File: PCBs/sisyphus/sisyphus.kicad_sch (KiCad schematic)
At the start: 65 parts, among them J1 USB_C_Receptacle_USB2.0_14P, J2 AUX USB, J3 Conn_01x02, J4 Speaker, J5 SWD, J6 RGB_CONN, J7 Keyboard, J8 Light sensor, J9 Battery, U1 NCP1117-3.3_SOT223, U2 USBLC6-2P6, U3 W25Q128JVS, U4 MAX98357A, U5 RP2040, U7 BQ25619, Y1 ABM8-272-T3

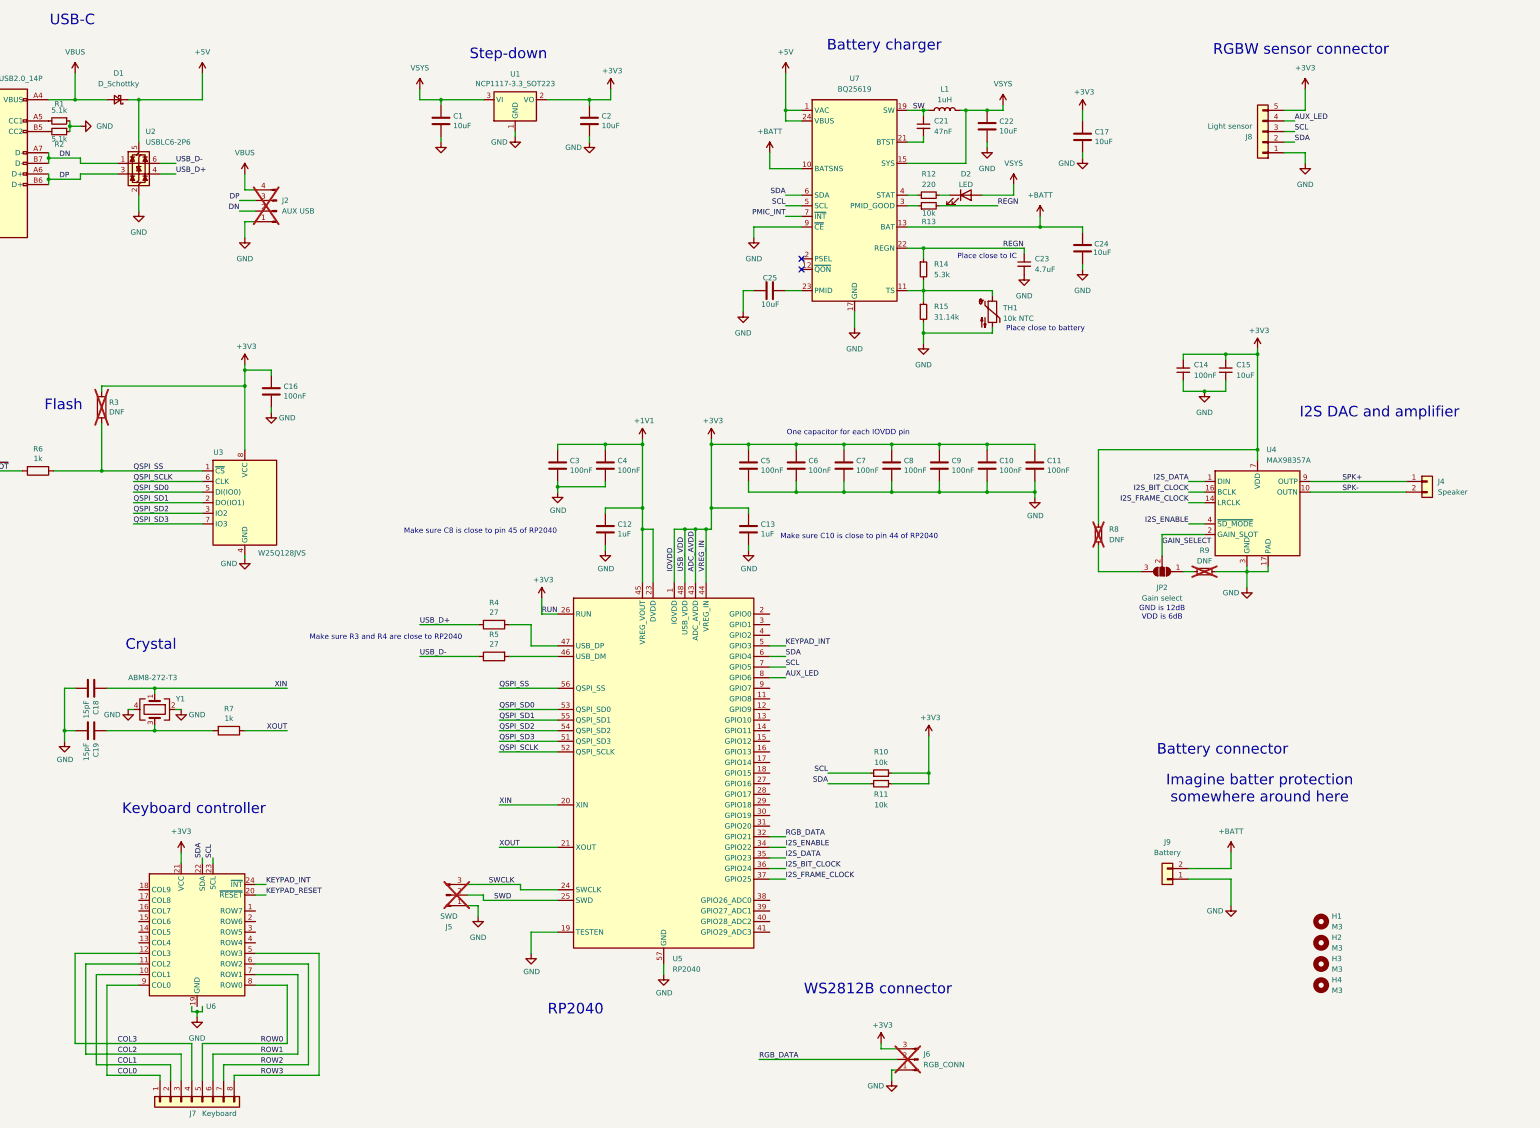
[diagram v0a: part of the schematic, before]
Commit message: Major PCB update
I won't even bother commenting it
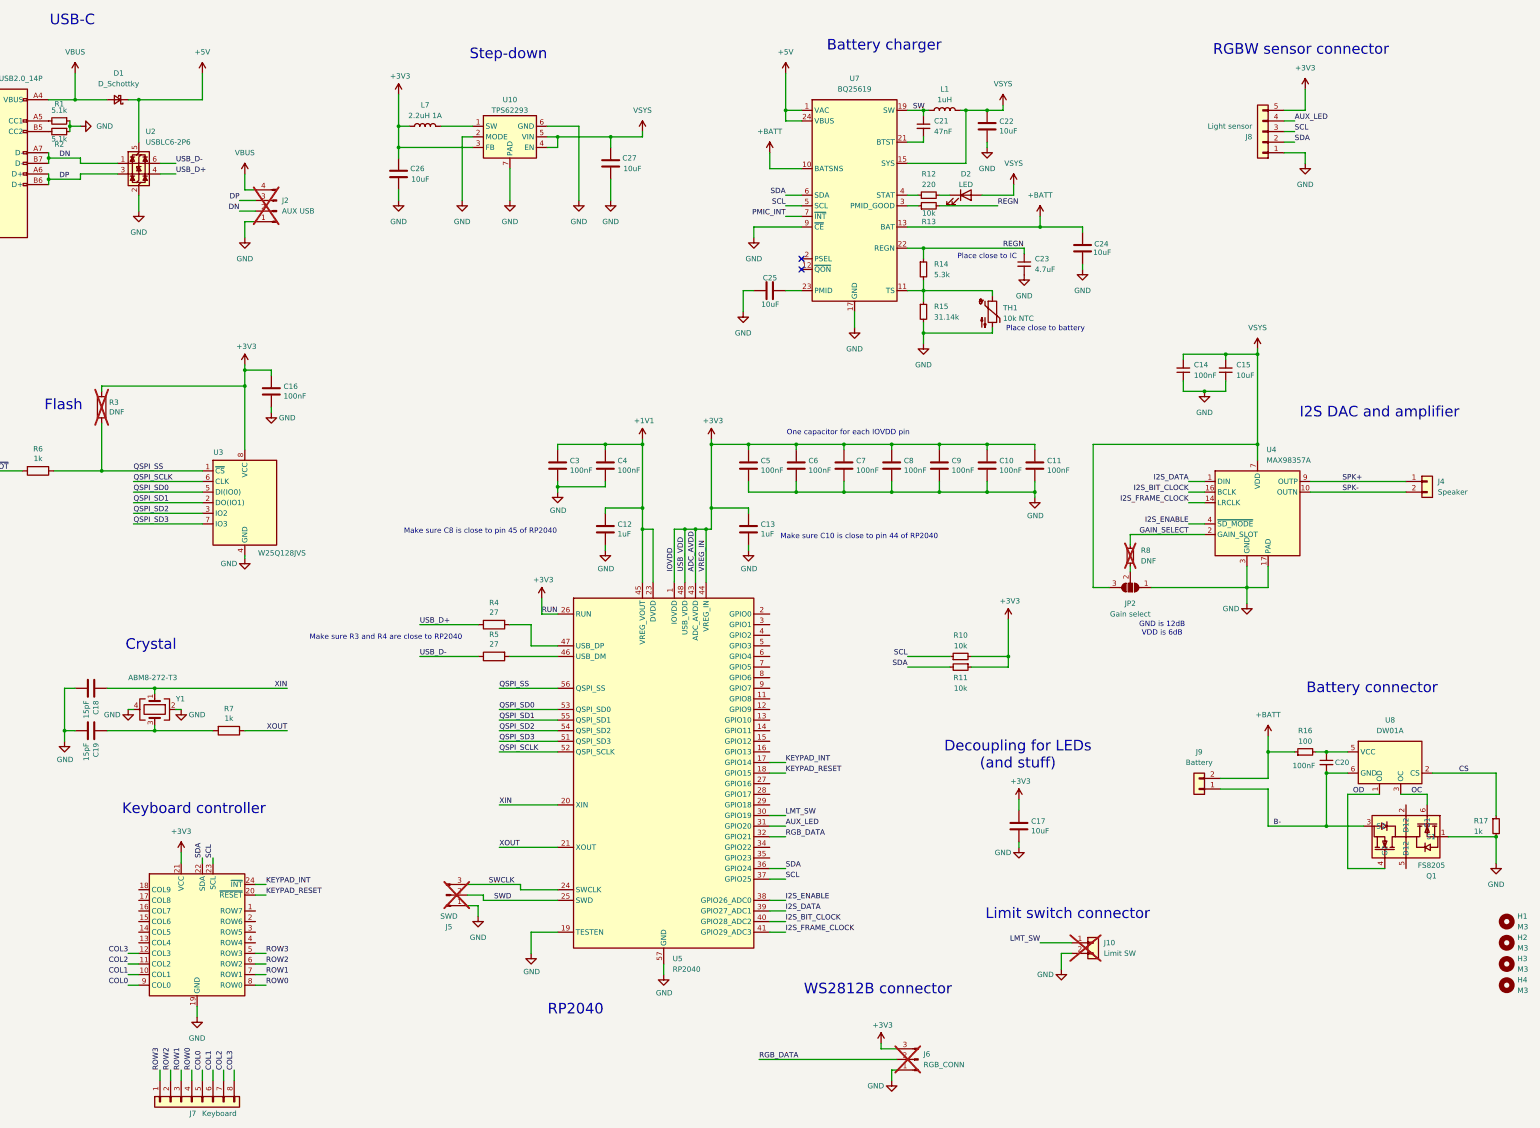
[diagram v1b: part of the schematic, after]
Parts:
- removed C1, C2: 10uF, Capacitor_SMD:C_0805_2012Metric, symbol Device:C
- removed R9: DNF, Resistor_SMD:R_0402_1005Metric, symbol Device:R_Small
- removed U1: NCP1117-3.3_SOT223, Package_TO_SOT_SMD:SOT-223-3_TabPin2, symbol Regulator_Linear:NCP1117-3.3_SOT223
- added C20: 100nF, Capacitor_SMD:C_0402_1005Metric, symbol Device:C_Small
- added C26, C27: 10uF, Capacitor_SMD:C_0402_1005Metric, symbol Device:C
- added J10: Limit SW, Connector_PinSocket_2.54mm:PinSocket_1x02_P2.54mm_Vertical, symbol Connector_Generic:Conn_01x02
- added L7: 2.2uH 1A, Inductor_SMD:L_0603_1608Metric, symbol Device:L
- added Q1: FS8205, Package_TO_SOT_SMD:SOT-23-6, symbol easyeda2kicad:FS8205
- added R16: 100, Resistor_SMD:R_0402_1005Metric, symbol Device:R_Small
- added R17: 1k, Resistor_SMD:R_0402_1005Metric, symbol Device:R_Small
- added U10: TPS62293, Package_SON:WSON-6-1EP_2x2mm_P0.65mm_EP1x1.6mm_ThermalVias, symbol Sisyphus:TPS62293
- added U8: DW01A, Package_TO_SOT_SMD:SOT-23-6, symbol Battery_Management:DW01A
- C15, C17, C22, C24, C25: footprint Capacitor_SMD:C_0805_2012Metric -> Capacitor_SMD:C_0402_1005Metric
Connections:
- net +3V3: now also C26.1, L7.1, U10.3 (FB); no longer C14.2, C15.2, R8.1, U4.7 (VDD), U4.8 (VDD)
- net +BATT: now also R16.1
- net AUX_LED: now also U5.31 (GPIO20); no longer U5.8 (GPIO6)
- net COL0: now also J7.5 (Pin_5); no longer J7.1 (Pin_1)
- net COL1: now also J7.6 (Pin_6); no longer J7.2 (Pin_2)
- net COL2: now also J7.7 (Pin_7); no longer J7.3 (Pin_3)
- net COL3: now also J7.8 (Pin_8); no longer J7.4 (Pin_4)
- net GAIN_SELECT: now also R8.1; no longer JP2.2 (C)
- net GND: now also JP2.1 (A), U6.19 (GND), U6.25 (PAD), C26.2, C27.2, J10.2 (Pin_2), Q1.1 (S1), R17.2, U10.2 (MODE), U10.6 (GND), U10.7 (PAD); no longer J9.1 (Pin_1)
- net I2S_BIT_CLOCK: now also U5.40 (GPIO28_ADC2); no longer U5.36 (GPIO24)
- net I2S_DATA: now also U5.39 (GPIO27_ADC1); no longer U5.35 (GPIO23)
- net I2S_ENABLE: now also U5.38 (GPIO26_ADC0); no longer U5.34 (GPIO22)
- net I2S_FRAME_CLOCK: now also U5.41 (GPIO29_ADC3); no longer U5.37 (GPIO25)
- net KEYPAD_INT: now also U5.17 (GPIO14); no longer U5.5 (GPIO3)
- net KEYPAD_RESET: now also U5.18 (GPIO15)
- net ROW0: now also J7.4 (Pin_4); no longer J7.5 (Pin_5)
- net ROW1: now also J7.3 (Pin_3); no longer J7.6 (Pin_6)
- net ROW2: now also J7.2 (Pin_2); no longer J7.7 (Pin_7)
- net ROW3: now also J7.1 (Pin_1); no longer J7.8 (Pin_8)
- net SCL: now also U5.37 (GPIO25); no longer U5.7 (GPIO5)
- net SDA: now also U5.36 (GPIO24); no longer U5.6 (GPIO4)
- net VSYS: now also C14.2, C15.2, JP2.3 (B), U4.7 (VDD), U4.8 (VDD), C27.1, U10.4 (EN), U10.5 (VIN)
- net at R8.2: now also JP2.2 (C); no longer JP2.3 (B)
- net LMT_SW: now reaches U5.30 (GPIO19)
- net LMT_SW: now also J10.1 (Pin_1)
- new net: C20.1, R16.2, U8.5 (VCC)
- new net: L7.2, U10.1 (SW)
- new net B-: C20.2, J9.1 (Pin_1), Q1.3 (S2), U8.6 (GND)
- new net CS: R17.1, U8.2 (CS)
- new net OC: Q1.6 (G1), U8.3 (OC)
- new net OD: Q1.4 (G2), U8.1 (OD)
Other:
- note added: "Decoupling for LEDs (and stuff)"
- note added: "Limit switch connector"
- note removed: "Imagine batter protection somewhere around here"
- moved on the sheet: C17, H1, H2, H3, H4, J9, JP2, R10, R11, R8
